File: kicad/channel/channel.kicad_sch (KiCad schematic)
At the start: 34 parts, among them J1 Conn_01x07_Male, J2 Conn_01x01_Male, J3 Conn_01x01_Male, J4 Conn_01x01_Male, J5 Conn_01x01_Male, Q1 BC846B, Q2 IRF3205, Q3 IRF3205, Q4 BC846B, Q5 IRF3205, Q6 IRF3205, U1 LM324

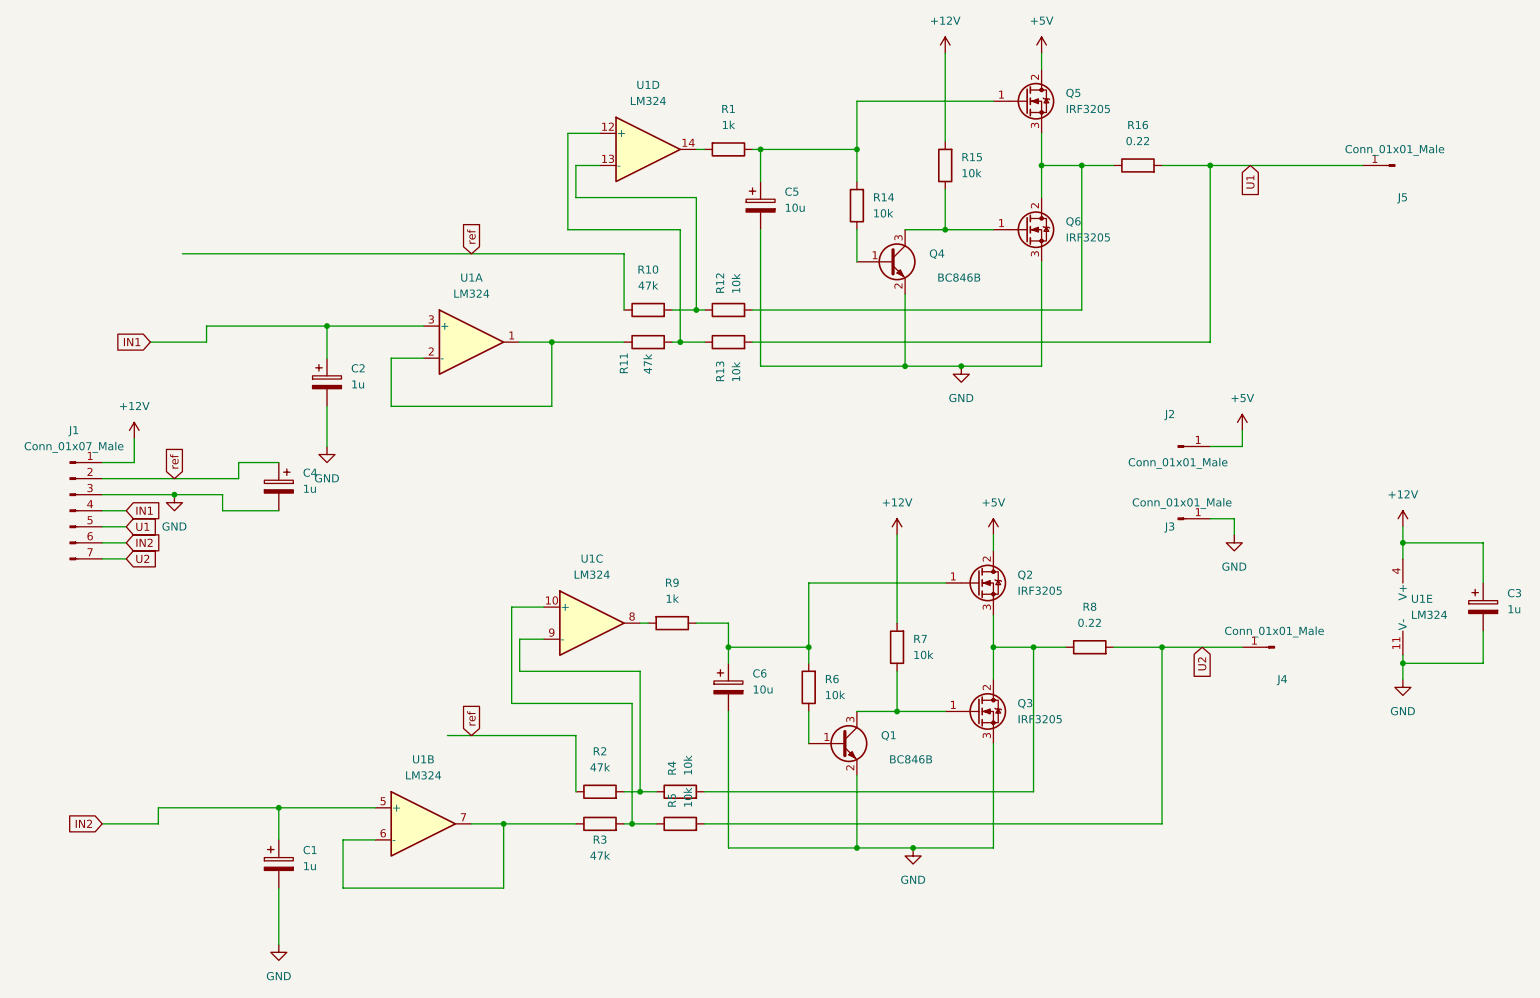
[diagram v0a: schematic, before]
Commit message: work on kicad
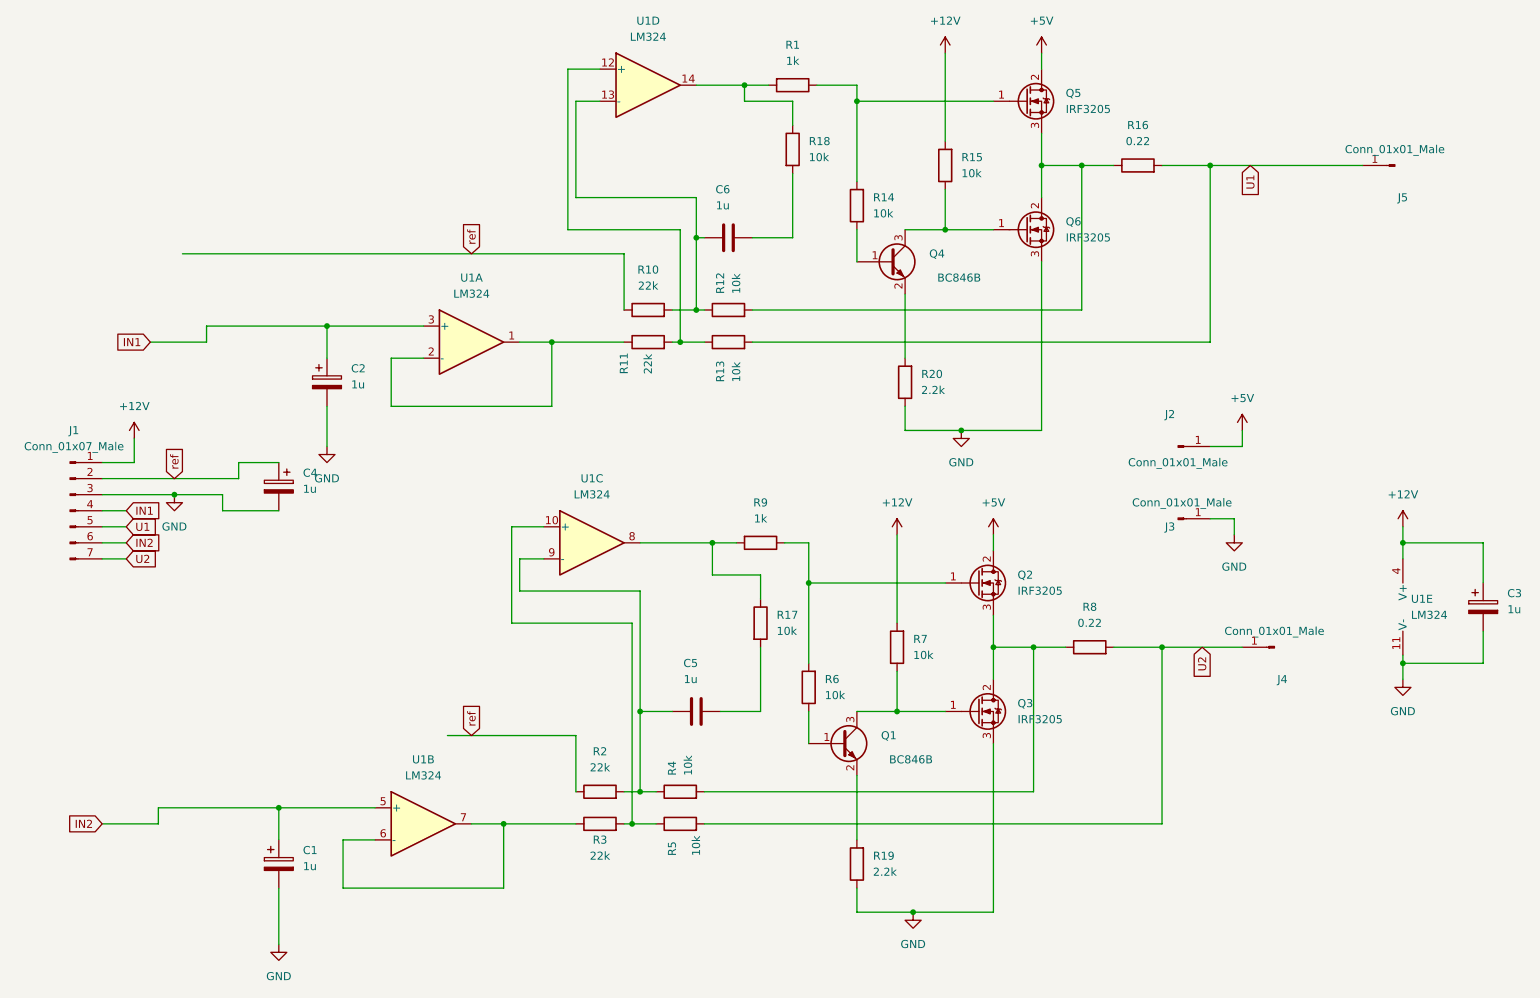
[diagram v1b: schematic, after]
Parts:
- removed C5, C6: 10u, Capacitor_SMD:CP_Elec_6.3x7.7, symbol Device:C_Polarized
- added C5, C6: 1u, Capacitor_SMD:C_0603_1608Metric, symbol Device:C
- added R17, R18: 10k, Resistor_SMD:R_1206_3216Metric, symbol Device:R
- added R19, R20: 2.2k, Resistor_SMD:R_1206_3216Metric, symbol Device:R
- R10, R11, R2, R3: value 47k -> 22k
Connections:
- net GND: now also R19.1, R20.1; no longer Q1.2 (E), Q4.2 (E)
- net at R1.2, U1.14: now also R18.1
- net at R2.2, R4.1, U1.9 (-): now also C5.1
- net at R9.2, U1.8: now also R17.1
- net at R10.2, R12.1, U1.13 (-): now also C6.1
- new net: C5.2, R17.2
- new net: Q1.2 (E), R19.2
- new net: C6.2, R18.2
- new net: Q4.2 (E), R20.2
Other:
- moved on the sheet: R1, R9, U1C, U1D
